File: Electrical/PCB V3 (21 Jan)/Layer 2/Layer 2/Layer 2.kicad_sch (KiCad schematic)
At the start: 92 parts, among them J1 XT60-M, J2 Conn_02x04_Odd_Even, J3 Conn_01x04, J5 Conn_01x02, Q1 AON6354, Q2 AON6354, Q3 AON6354, Q4 AON6354, SW2 SW_SPST, SW3 SW_SPST, U1 VNH5019ATR-E, U12 VNH5019ATR-E, U2 TPS5430DDAG4, U3 TPS5430DDAG4, U4 XT30UPB-M, U5 VNH5019ATR-E, U6 XT30UPB-M, U7 XT30UPB-M, U8 XT30UPB-M, U9 VNH5019ATR-E

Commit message: am i done im tired
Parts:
- J2: footprint Connector_JST:JST_EH_B8B-EH-A_1x08_P2.50mm_Vertical -> Connector_JST:JST_EH_B10B-EH-A_1x10_P2.50mm_Vertical
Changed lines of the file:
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@@
 			)
 		)
-		(property "Footprint" "Connector_JST:JST_EH_B8B-EH-A_1x08_P2.50mm_Vertical"
+		(property "Footprint" "Connector_JST:JST_EH_B10B-EH-A_1x10_P2.50mm_Vertical"
 			(at 110.49 238.76 0)
 			(effects

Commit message: did some touching up made traces less cursed with gnd fills in between and made schmeatics look better with aligned boxes
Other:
- note added: "2-Chairs."
- note added: "27 Febuary 2025"
- note added: "L1 Connections"
- note added: "L3 connection"
- note added: "Layer 2"
- note added: "Pull Up/ Down for Motor Drivers"
- note added: "V3"
- note removed: "L1 JST"
- note removed: "L3 JST"
- note removed: "Pull Up"
- moved on the sheet: A1, C1, C10, C14, C2, C3, C4, C5, C6, C7, C8, D1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

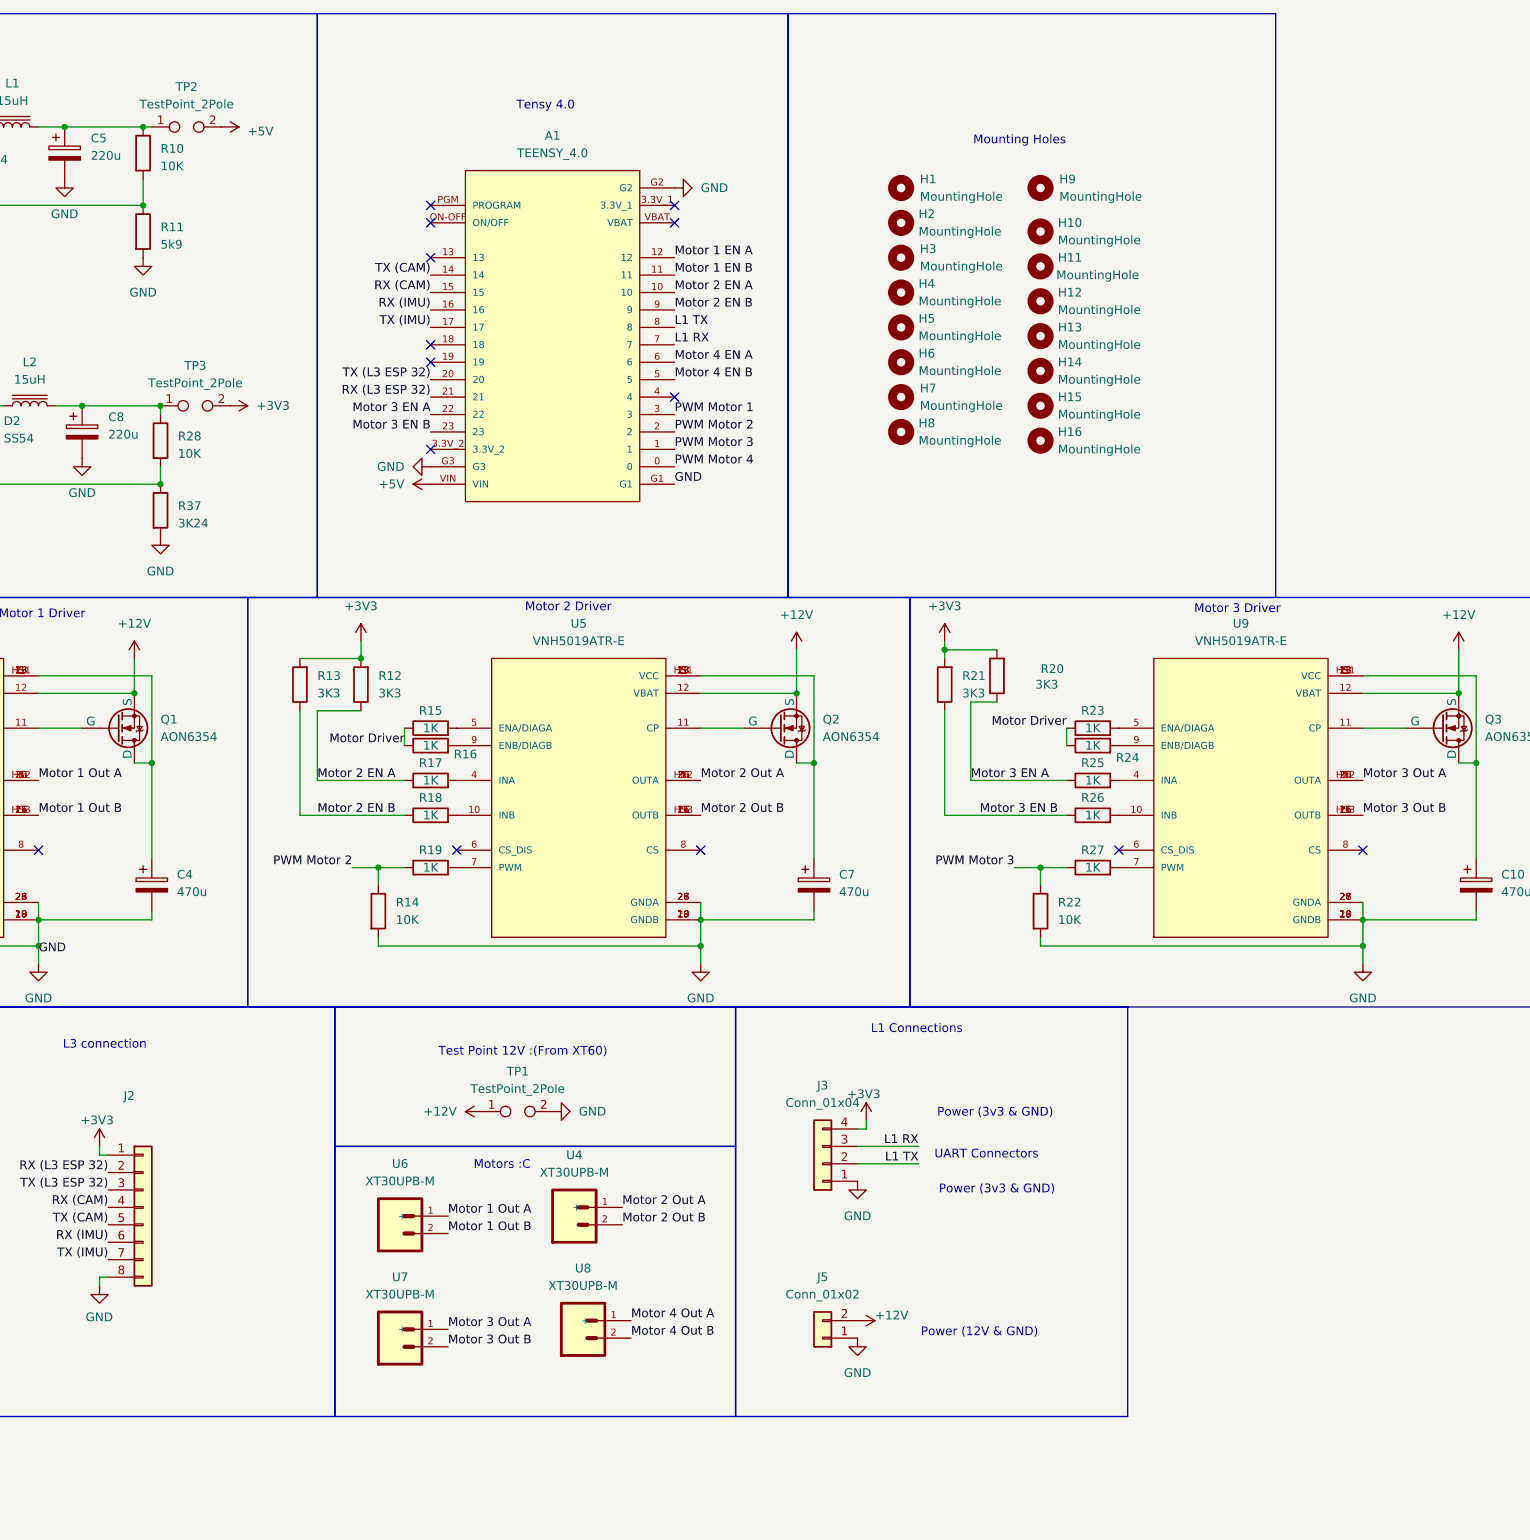
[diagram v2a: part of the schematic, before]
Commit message: m
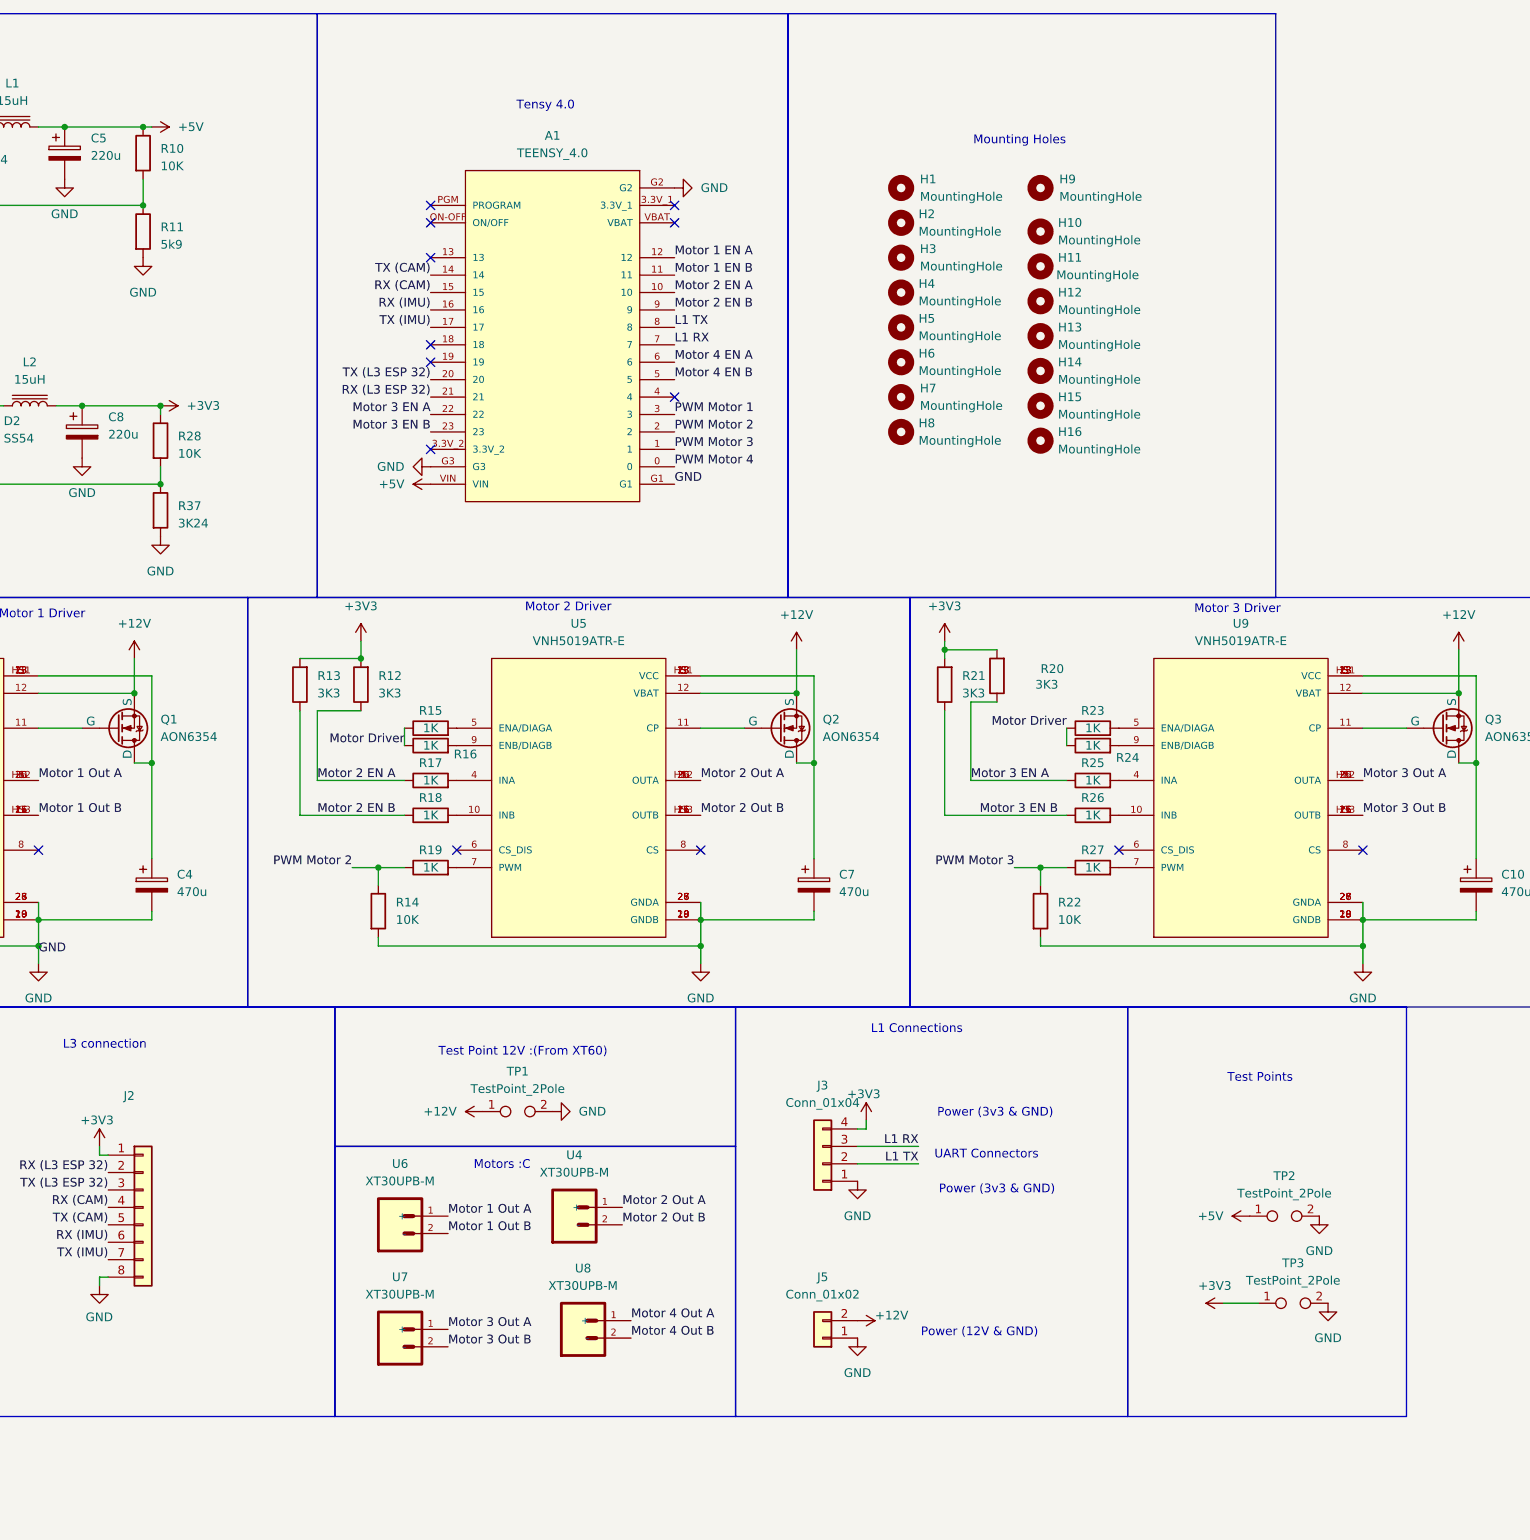
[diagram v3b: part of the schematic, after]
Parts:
- TP1, TP2, TP3: footprint Custom Testpointverycool:testpoint_2pad_2-chairs. -> Custom Testpointverycool:14 AWG Testpoint
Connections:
- net +3V3: now also C8.1, L2.2, R28.1, TP3.1; no longer TP3.2
- net +5V: now also C5.1, L1.2, R10.1, TP2.1; no longer TP2.2
- net GND: now also TP2.2, TP3.2
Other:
- note added: "Test Points"
- moved on the sheet: TP2, TP3

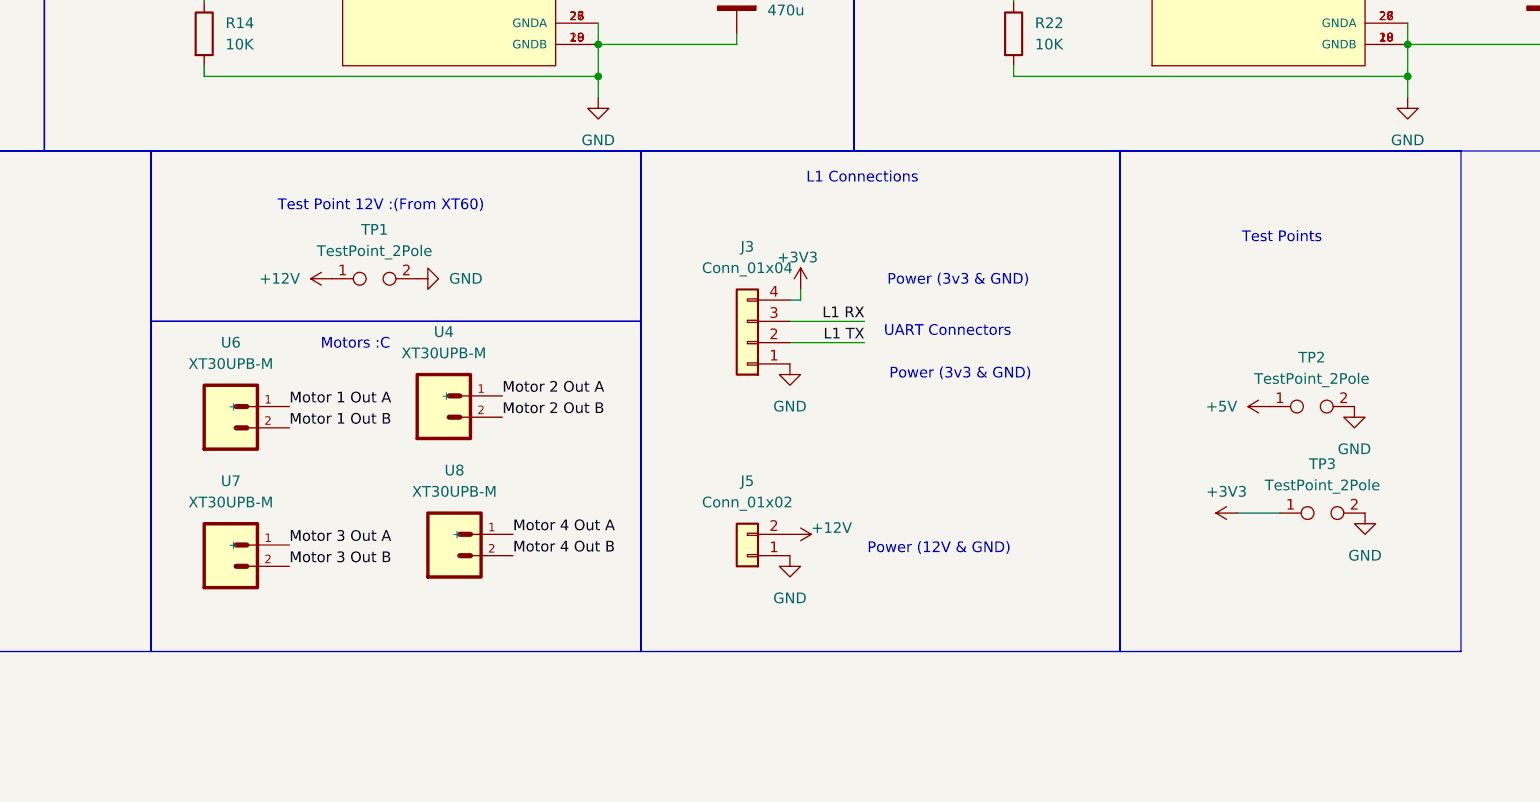
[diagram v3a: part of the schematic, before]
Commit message: ok testpoints
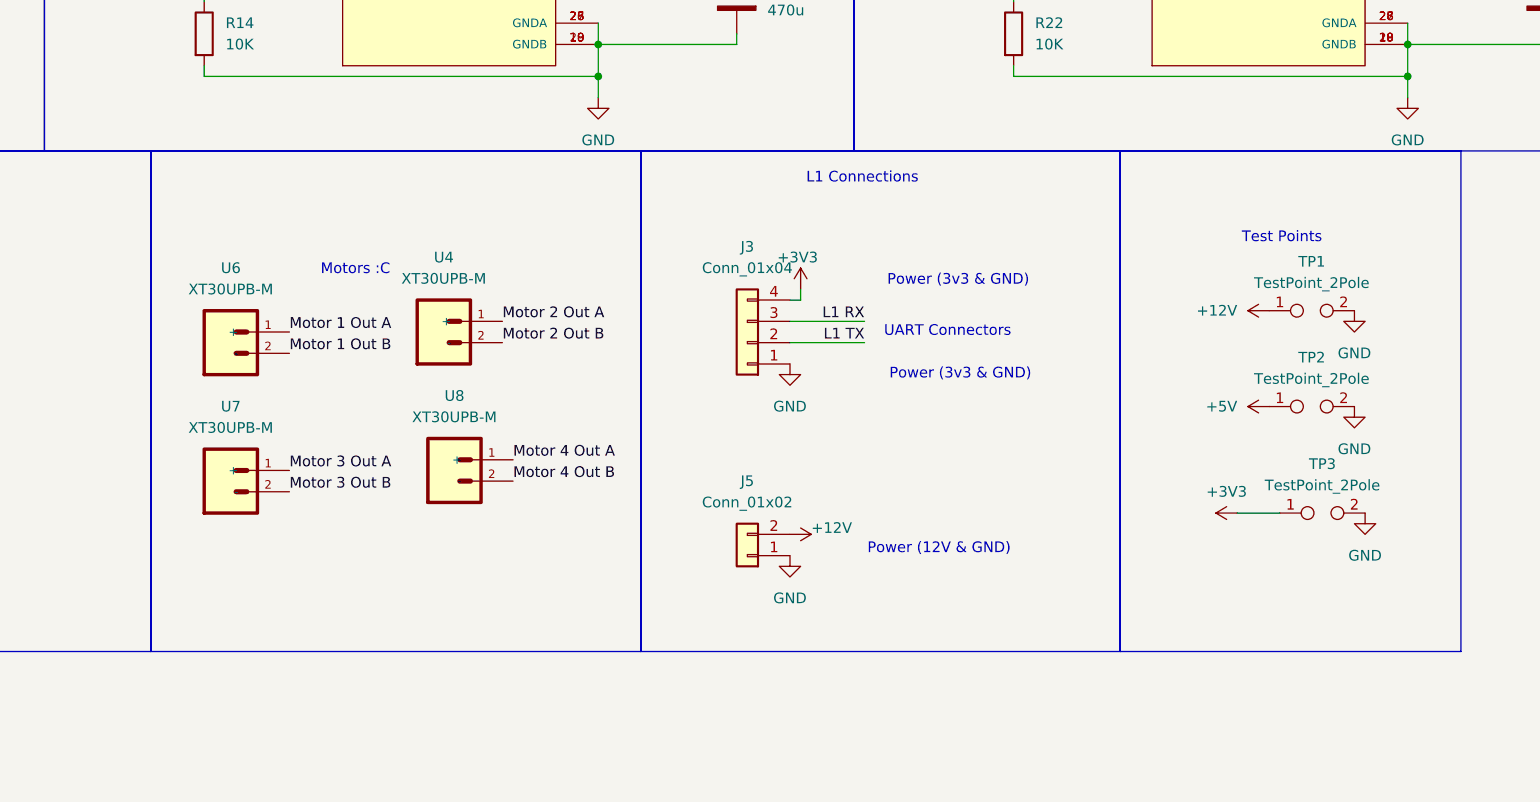
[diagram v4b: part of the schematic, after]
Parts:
- TP1, TP3: footprint Custom Testpointverycool:14 AWG Testpoint -> Custom Testpointverycool:14 AWG Testpoint (Vertical)
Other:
- note removed: "Test Point 12V :(From XT60)"
- moved on the sheet: TP1, U4, U6, U7, U8

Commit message: erm moved 2 drivers flip
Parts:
- TP2: footprint Custom Testpointverycool:14 AWG Testpoint -> Custom Testpointverycool:14 AWG Testpoint (Vertical)
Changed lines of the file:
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@@
 			)
 		)
-		(property "Footprint" "Custom Testpointverycool:14 AWG Testpoint"
+		(property "Footprint" "Custom Testpointverycool:14 AWG Testpoint (Vertical)"
 			(at 260.35 189.23 0)
 			(effects

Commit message: fixed l2
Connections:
- net GND: no longer U3.6 (GND), U3.9 (POWER_PAD)
- net  RX (L3 ESP 32) renamed RX (L3 ESP 32)
- net  TX (L3 ESP 32) renamed TX (L3 ESP 32)
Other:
- moved on the sheet: C1, C10, C14, C2, C3, C4, C5, C6, C7, C8, D1, D2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
